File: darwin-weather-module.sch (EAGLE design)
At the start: 14 parts, among them U1 P82B715SOIC

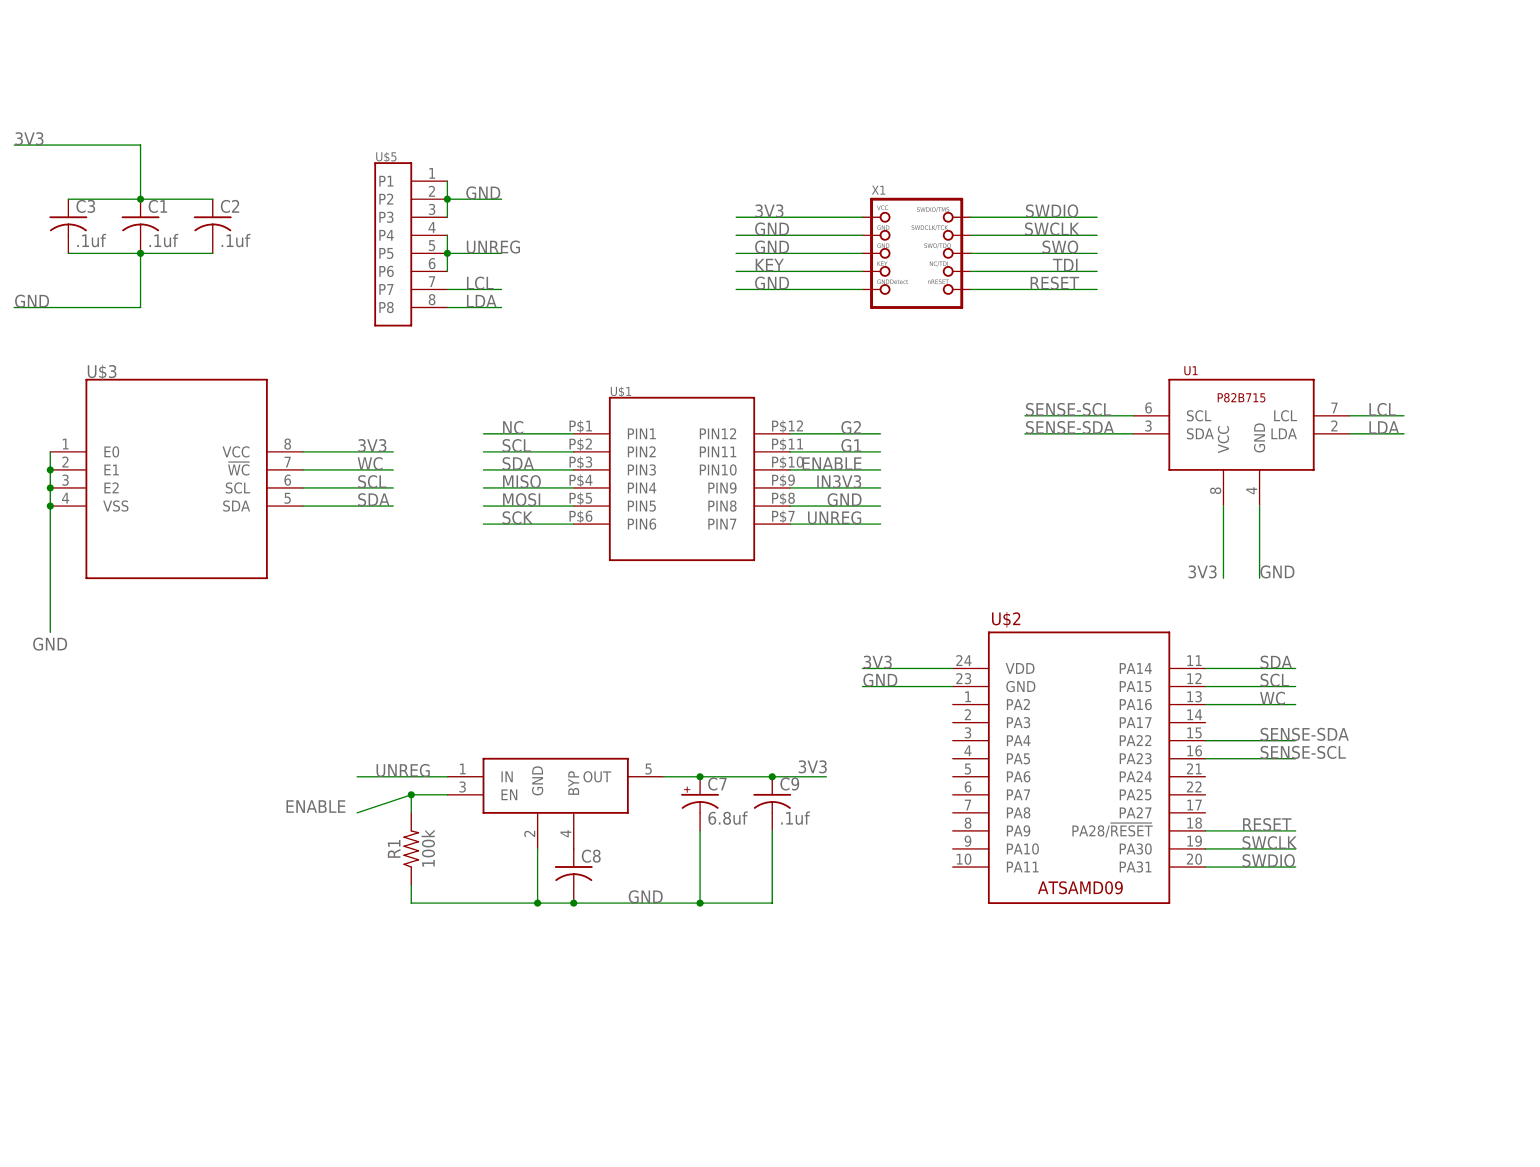
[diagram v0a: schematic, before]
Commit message: Schematic Cleanup
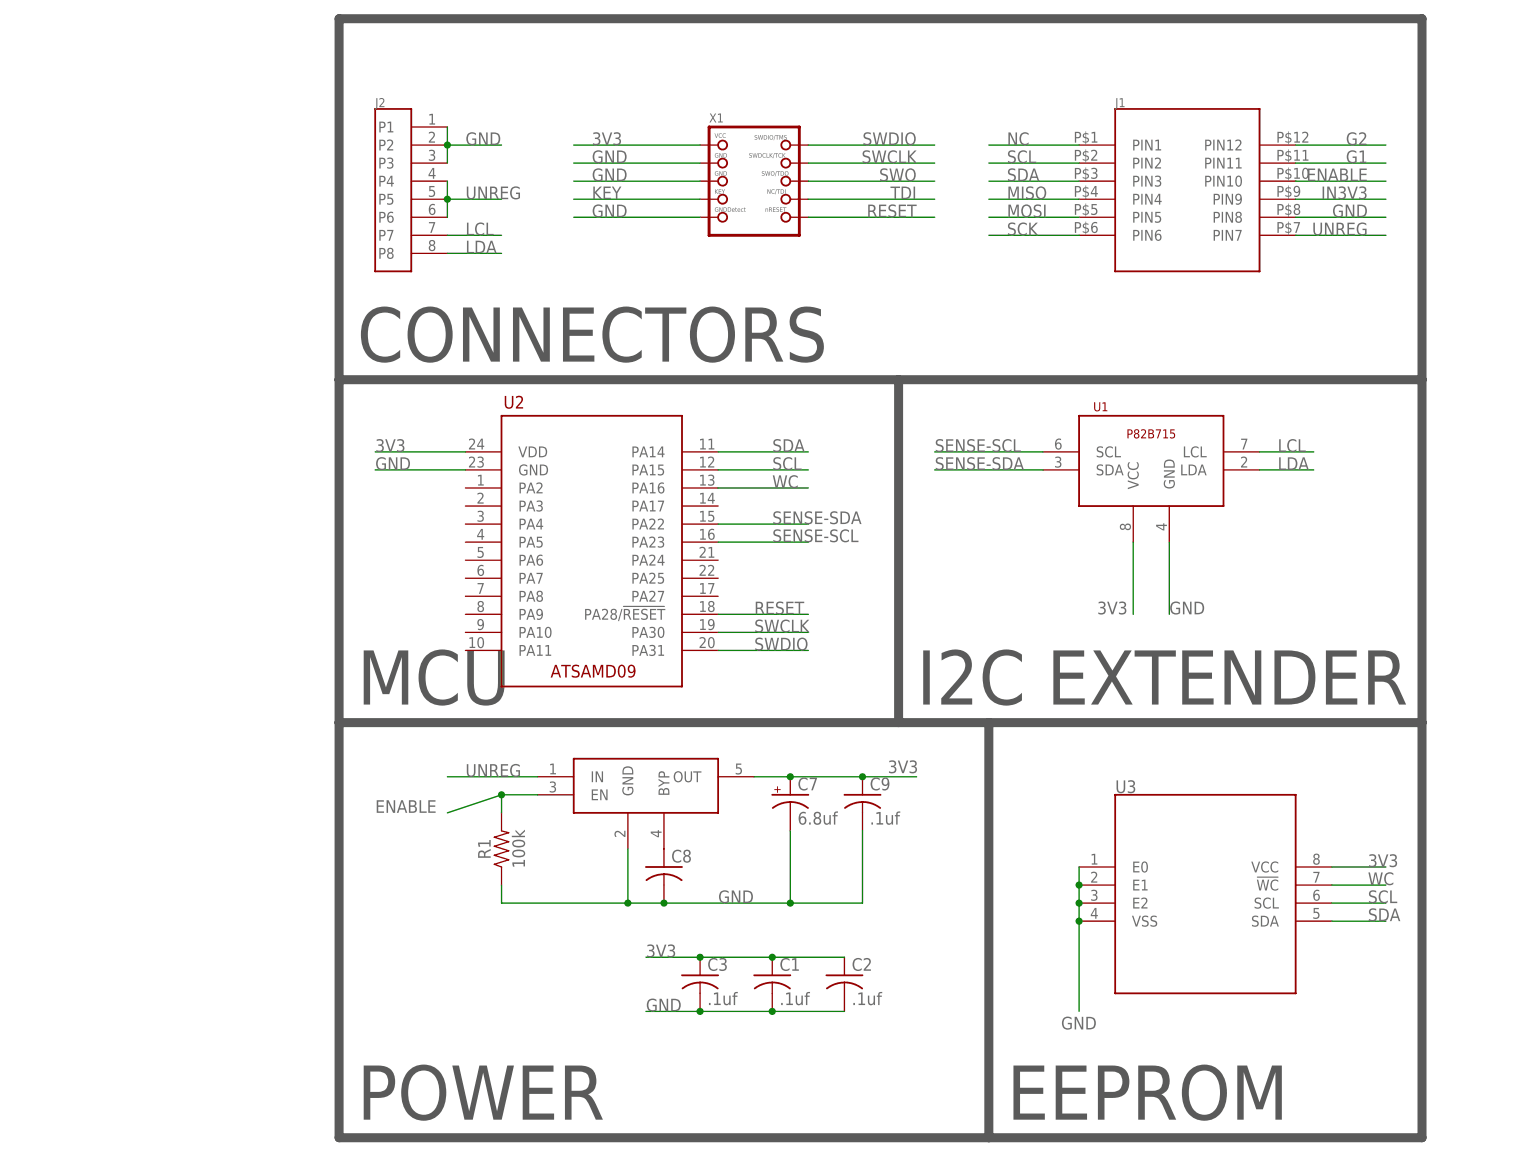
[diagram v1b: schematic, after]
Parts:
- removed U$1: 2X6-HEADERS, Conservify:2X6-HEADERS
- removed U$2: ATSAMD09, Conservify:ATSAMD09
- removed U$3: M24C02-WMN6TP, Conservify:M24C02-WMN6TP
- removed U$5: 95501-6889VERT, Conservify:95501-6889VERT
- added J1: 2X6-HEADERS, Conservify:2X6-HEADERS
- added J2: 95501-6889VERT, Conservify:95501-6889VERT
- added U2: ATSAMD09, Conservify:ATSAMD09
- added U3: M24C02-WMN6TP, Conservify:M24C02-WMN6TP
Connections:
- net 3V3: now also U2.VDD, U3.VCC; no longer U$2.VDD, U$3.VCC
- net ENABLE: now also J1.PIN10; no longer U$1.PIN10
- net G1: now also J1.PIN11; no longer U$1.PIN11
- net G2: now also J1.PIN12; no longer U$1.PIN12
- net GND: now also J1.PIN8, J2.P1, J2.P2, J2.P3, U2.GND, U3.E0, U3.E1, U3.E2, U3.VSS; no longer U$1.PIN8, U$2.GND, U$3.E0, U$3.E1, U$3.E2, U$3.VSS, U$5.P1, U$5.P2, U$5.P3
- net IN3V3: now also J1.PIN9; no longer U$1.PIN9
- net LCL: now also J2.P7; no longer U$5.P7
- net LDA: now also J2.P8; no longer U$5.P8
- net MISO: now also J1.PIN4; no longer U$1.PIN4
- net MOSI: now also J1.PIN5; no longer U$1.PIN5
- net NC: now also J1.PIN1; no longer U$1.PIN1
- net RESET: now also U2.PA28/!RESET; no longer U$2.PA28/!RESET
- net SCK: now also J1.PIN6; no longer U$1.PIN6
- net SCL: now also J1.PIN2, U2.PA15, U3.SCL; no longer U$1.PIN2, U$2.PA15, U$3.SCL
- net SDA: now also J1.PIN3, U2.PA14, U3.SDA; no longer U$1.PIN3, U$2.PA14, U$3.SDA
- net SENSE-SCL: now also U2.PA23; no longer U$2.PA23
- net SENSE-SDA: now also U2.PA22; no longer U$2.PA22
- net SWCLK: now also U2.PA30; no longer U$2.PA30
- net SWDIO: now also U2.PA31; no longer U$2.PA31
- net UNREG: now also J1.PIN7, J2.P4, J2.P5, J2.P6; no longer U$1.PIN7, U$5.P4, U$5.P5, U$5.P6
- net WC: now also U2.PA16, U3.!WC; no longer U$2.PA16, U$3.!WC
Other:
- note added: "CONNECTORS"
- note added: "EEPROM"
- note added: "I2C EXTENDER"
- note added: "MCU"
- note added: "POWER"
- moved on the sheet: C1, C2, C3, C7, C8, C9, R1, U1, X1
